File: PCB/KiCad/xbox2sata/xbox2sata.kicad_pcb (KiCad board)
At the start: 4 copper layers, 85 x 52.1 mm, 21 parts, among them J1 61203921621, J2 67800-8025, J3 90151-2140, U1 88SA8052, Y1 ABLS-25.000MHZ-B4-F-T

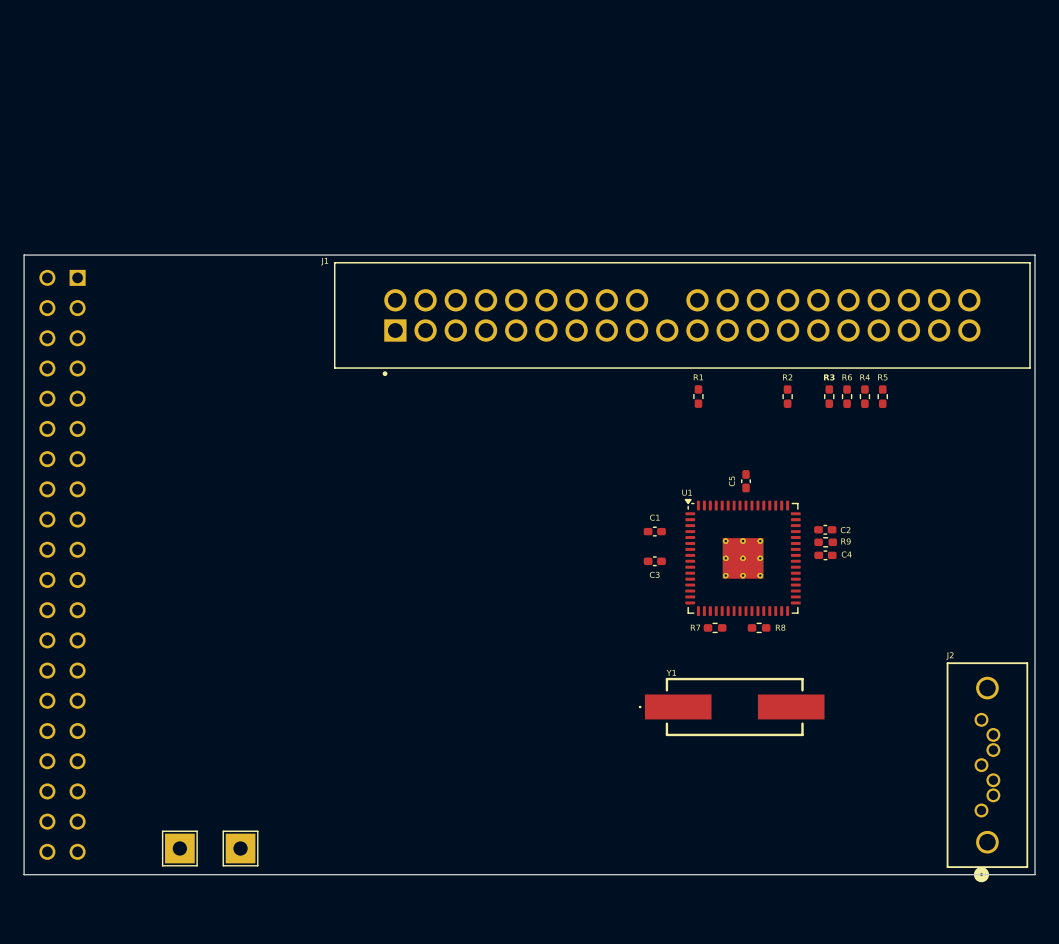
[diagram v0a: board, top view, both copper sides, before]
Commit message: KiCad update
Added to schematic and pcb
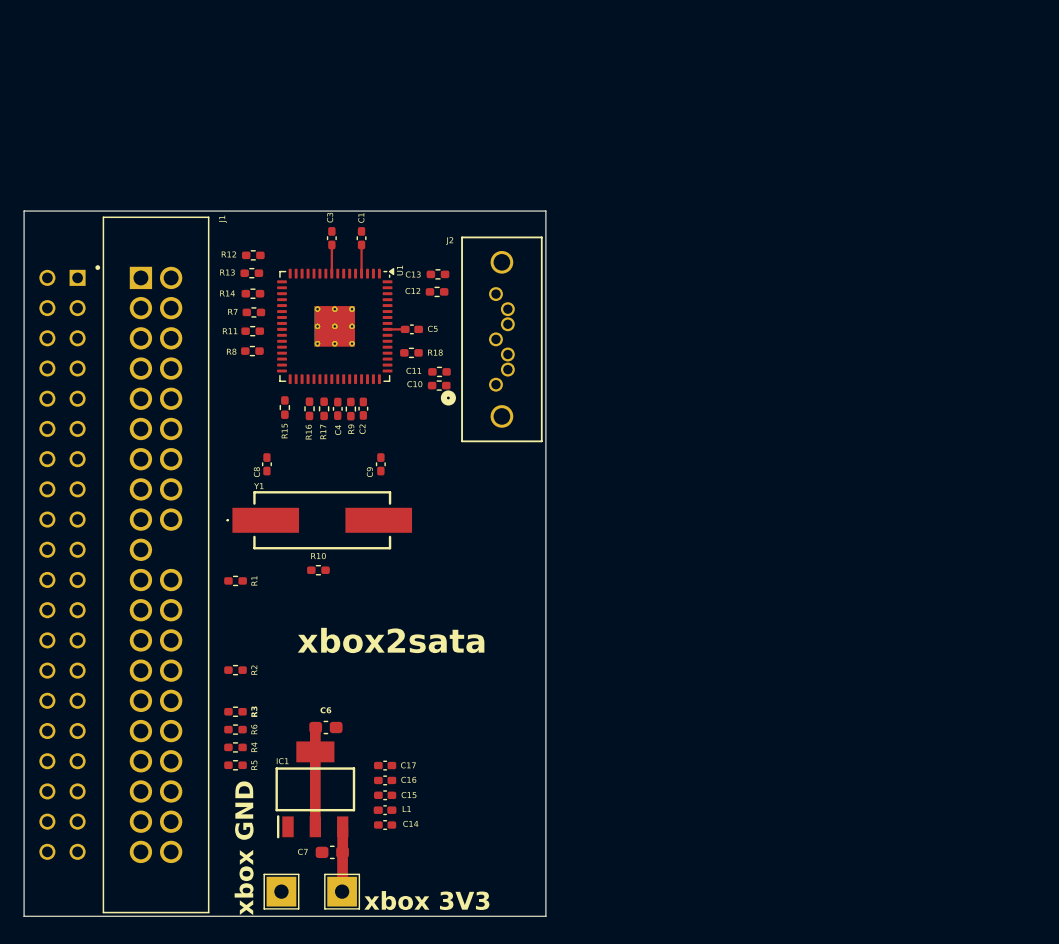
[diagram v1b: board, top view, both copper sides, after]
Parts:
- added C10: 10nF, Resistor_SMD:R_0402_1005Metric_Pad0.72x0.64mm_HandSolder, F.Cu at (123.4, 74.5)
- added C11: 10nF, Resistor_SMD:R_0402_1005Metric_Pad0.72x0.64mm_HandSolder, F.Cu at (123.4, 73.3)
- added C12: 10nF, Resistor_SMD:R_0402_1005Metric_Pad0.72x0.64mm_HandSolder, F.Cu at (123.2, 66.6)
- added C13: 10nF, Resistor_SMD:R_0402_1005Metric_Pad0.72x0.64mm_HandSolder, F.Cu at (123.3, 65.1)
- added C14: 10nF, Capacitor_SMD:C_0402_1005Metric_Pad0.74x0.62mm_HandSolder, F.Cu at (118.9, 111.4)
- added C15: 100nF, Capacitor_SMD:C_0402_1005Metric_Pad0.74x0.62mm_HandSolder, F.Cu at (118.9, 108.9)
- added C16: 100nF, Capacitor_SMD:C_0402_1005Metric_Pad0.74x0.62mm_HandSolder, F.Cu at (118.9, 107.7)
- added C17: 10nF, Capacitor_SMD:C_0402_1005Metric_Pad0.74x0.62mm_HandSolder, F.Cu at (118.9, 106.4)
- added C6: 1uF, Capacitor_SMD:C_0603_1608Metric_Pad1.08x0.95mm_HandSolder, F.Cu at (113.9, 103.2)
- added C7: 1uF, Capacitor_SMD:C_0603_1608Metric_Pad1.08x0.95mm_HandSolder, F.Cu at (114.4, 113.7)
- added C8: 18pF, Capacitor_SMD:C_0402_1005Metric_Pad0.74x0.62mm_HandSolder, F.Cu at (108.9, 81.1)
- added C9: 18pF, Capacitor_SMD:C_0402_1005Metric_Pad0.74x0.62mm_HandSolder, F.Cu at (118.5, 81.1)
- added IC1: TLV1117LV12DCYR, xbox2sata:SOT230P700X180-4N, F.Cu at (113.0, 108.4)
- added L1: L, Inductor_SMD:L_0402_1005Metric_Pad0.77x0.64mm_HandSolder, F.Cu at (118.9, 110.2)
- added R10: 1M, Resistor_SMD:R_0402_1005Metric_Pad0.72x0.64mm_HandSolder, F.Cu at (113.2, 90.0)
- added R11: 100, Resistor_SMD:R_0402_1005Metric_Pad0.72x0.64mm_HandSolder, F.Cu at (107.7, 69.9)
- added R12: 10K, Resistor_SMD:R_0402_1005Metric_Pad0.72x0.64mm_HandSolder, F.Cu at (107.8, 63.5)
- added R13: 10K, Resistor_SMD:R_0402_1005Metric_Pad0.72x0.64mm_HandSolder, F.Cu at (107.6, 65.0)
- added R14: 10K, Resistor_SMD:R_0402_1005Metric_Pad0.72x0.64mm_HandSolder, F.Cu at (107.7, 66.8)
- added R15: 4.7K, Resistor_SMD:R_0402_1005Metric_Pad0.72x0.64mm_HandSolder, F.Cu at (110.4, 76.3)
- added R16: 10K, Resistor_SMD:R_0402_1005Metric_Pad0.72x0.64mm_HandSolder, F.Cu at (112.5, 76.4)
- added R17: 10K, Resistor_SMD:R_0402_1005Metric_Pad0.72x0.64mm_HandSolder, F.Cu at (113.7, 76.4)
- added R18: 10K, Resistor_SMD:R_0402_1005Metric_Pad0.72x0.64mm_HandSolder, F.Cu at (121.1, 71.7)
- moved R5 62.6 mm to (106.3, 106.4), turned to 180 degrees
- moved R4 60.6 mm to (106.3, 104.9), turned to 0 degrees
- moved R6 58.6 mm to (106.3, 103.4), turned to 180 degrees
- moved R3 56.5 mm to (106.3, 101.9), turned to 0 degrees
- moved J2 54.3 mm to (128.2, 74.4)
- moved R2 51.8 mm to (106.3, 98.4), turned to 0 degrees
- moved J1 49.0 mm to (99.6, 89.6), turned to -90 degrees
- moved R8 48.5 mm to (107.7, 71.6), turned to 0 degrees
- moved R7 47.0 mm to (107.8, 68.3)
- moved C4 42.8 mm to (114.9, 76.4), turned to -90 degrees
- moved R1 41.9 mm to (106.3, 90.9), turned to 0 degrees
- moved R9 41.5 mm to (116.0, 76.4), turned to -90 degrees
- moved C2 40.2 mm to (117.0, 76.4), turned to -90 degrees
- moved U1 39.5 mm to (114.6, 69.5), turned to -90 degrees
- moved C3 38.4 mm to (114.4, 62.1), turned to 90 degrees
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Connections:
- J2 pad 1: unconnected-(J2-Pad1) -> GND
- J2 pad 2: unconnected-(J2-Pad2) -> Net-(C10-Pad2)
- J2 pad 3: unconnected-(J2-Pad3) -> Net-(C11-Pad2)
- J2 pad 4: unconnected-(J2-Pad4) -> GND
- J2 pad 5: unconnected-(J2-Pad5) -> Net-(C12-Pad2)
- J2 pad 6: unconnected-(J2-Pad6) -> Net-(C13-Pad2)
- J2 pad 7: unconnected-(J2-Pad7) -> GND
- J2 pad 8: unconnected-(J2-mount_1-Pad8) -> GND
- J2 pad 9: unconnected-(J2-mount_2-Pad9) -> GND
- U1 pad 37: T4 -> GND
- Y1 pad 1: unconnected-(Y1-Pad1) -> Net-(C8-Pad1)
- Y1 pad 2: unconnected-(Y1-Pad2) -> XTLIN
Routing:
- net 1V2: track 0.00 -> 12.3 mm
- net 3V3: track 0.00 -> 7.88 mm
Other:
- board size 85 x 52.1 mm -> 43.9 x 59.3 mm
- copper layers 4 -> 2
- board text added: "${REFERENCE}"
- board text added: "xbox 3V3"
- board text added: "xbox GND"
- board text added: "xbox2sata"

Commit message: slight changes to schematic
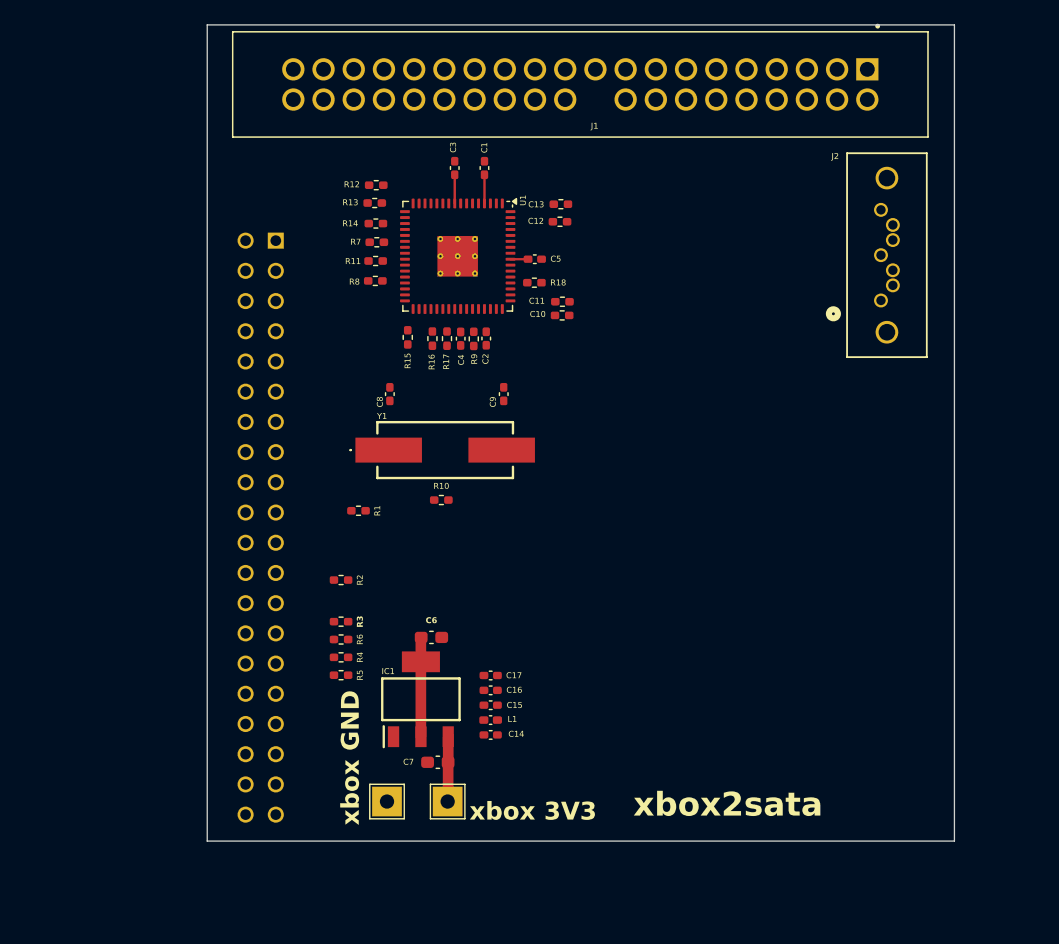
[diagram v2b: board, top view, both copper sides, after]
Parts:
- moved J1 53.9 mm to (135.3, 49.2), turned to 180 degrees
- moved J2 33.1 mm to (160.6, 67.3)
- moved J3 17.0 mm to (109.7, 62.3)
- moved C9 11.9 mm to (128.8, 75.2)
- moved R1 11.9 mm to (116.6, 85.0)
- moved R11 11.9 mm to (118.1, 64.0)
- moved R13 11.9 mm to (118.0, 59.1)
- moved R15 11.9 mm to (120.8, 70.4)
- moved R9 11.9 mm to (126.3, 70.5)
- moved R12 11.9 mm to (118.1, 57.6)
- moved C10 11.9 mm to (133.7, 68.6)
- moved C12 11.9 mm to (133.6, 60.7)
- moved R17 11.9 mm to (124.1, 70.5)
- moved Y1 11.9 mm to (123.9, 79.9)
- moved C1 11.9 mm to (127.2, 56.2)
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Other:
- board size 43.9 x 59.3 mm -> 62.8 x 68.6 mm
